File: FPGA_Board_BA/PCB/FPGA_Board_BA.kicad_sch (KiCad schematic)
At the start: 0 parts

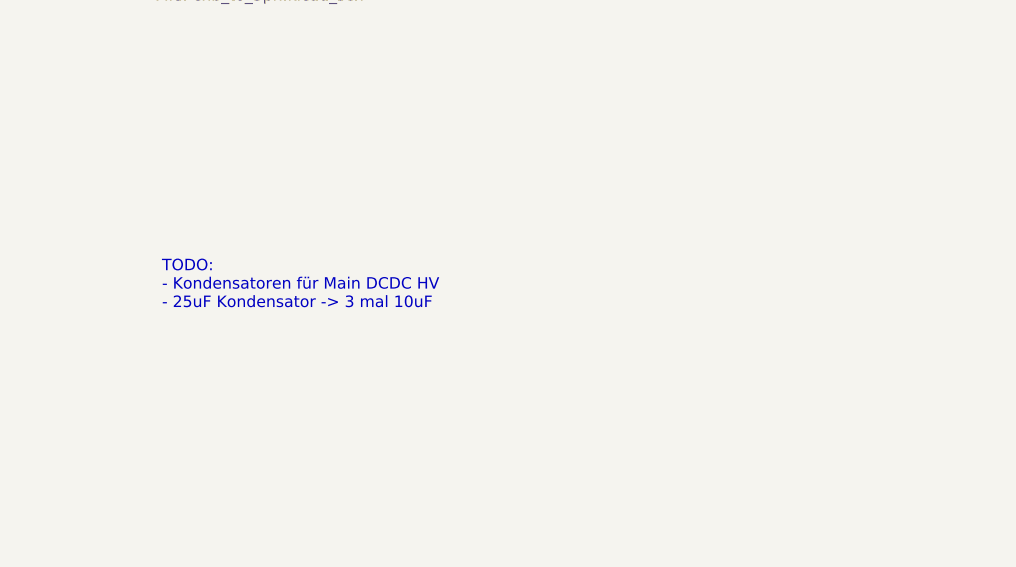
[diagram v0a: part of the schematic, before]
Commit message: schematic fixes after Leo Meeting
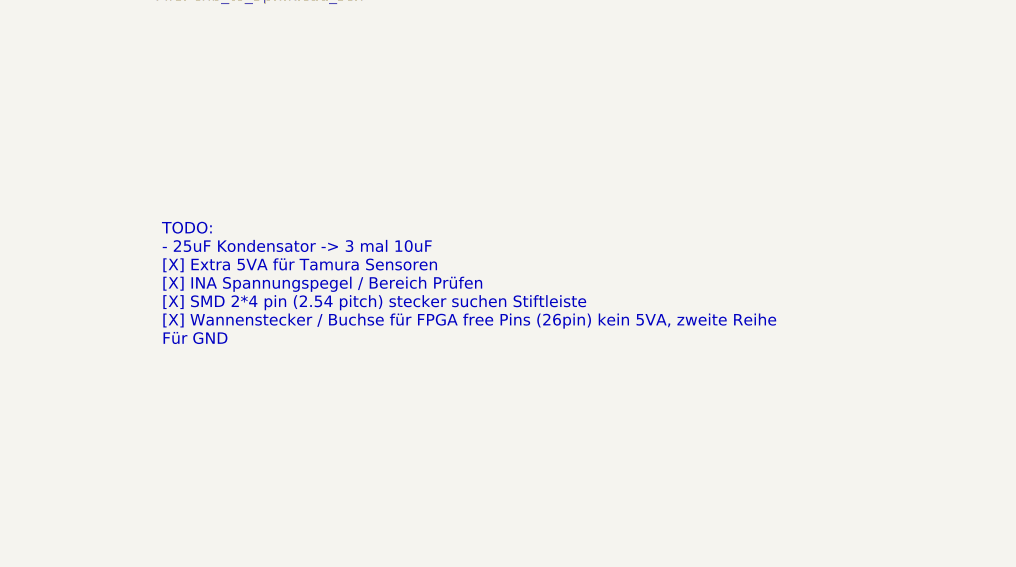
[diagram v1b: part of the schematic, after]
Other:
- note added: "TODO: - 25uF Kondensator -> 3 mal 10uF [X] Extra 5VA für Tamura Sensoren [X] INA Spannungspegel / Bereich Prüfen [X] SMD 2*4 pin (2.54 pitch) stecker suchen Stiftleiste [X] Wannenstecker / Buchse für FPGA free Pins (26pin) kein 5VA, zweite Reihe Für GND"
- note removed: "TODO: - Kondensatoren für Main DCDC HV - 25uF Kondensator -> 3 mal 10uF"
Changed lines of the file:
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@@
 	(generator_version "9.0")
 	(paper "A3")
-	(text "TODO:\n- Kondensatoren für Main DCDC HV\n- 25uF Kondensator -> 3 mal 10uF "
+	(text "TODO:\n- 25uF Kondensator -> 3 mal 10uF \n[X] Extra 5VA für Tamura Sensoren\n[X] INA Spannungspegel / Bereich Prüfen\n[X] SMD 2*4 pin (2.54 pitch) stecker suchen Stiftleiste\n[X] Wannenstecker / Buchse für FPGA free Pins (26pin) kein 5VA, zweite Reihe\nFür GND"
 		(exclude_from_sim no)
 		(at 328.422 239.268 0)
